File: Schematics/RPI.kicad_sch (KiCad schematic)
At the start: 7 parts, among them J1 RPi GPIO, U2 24LC256

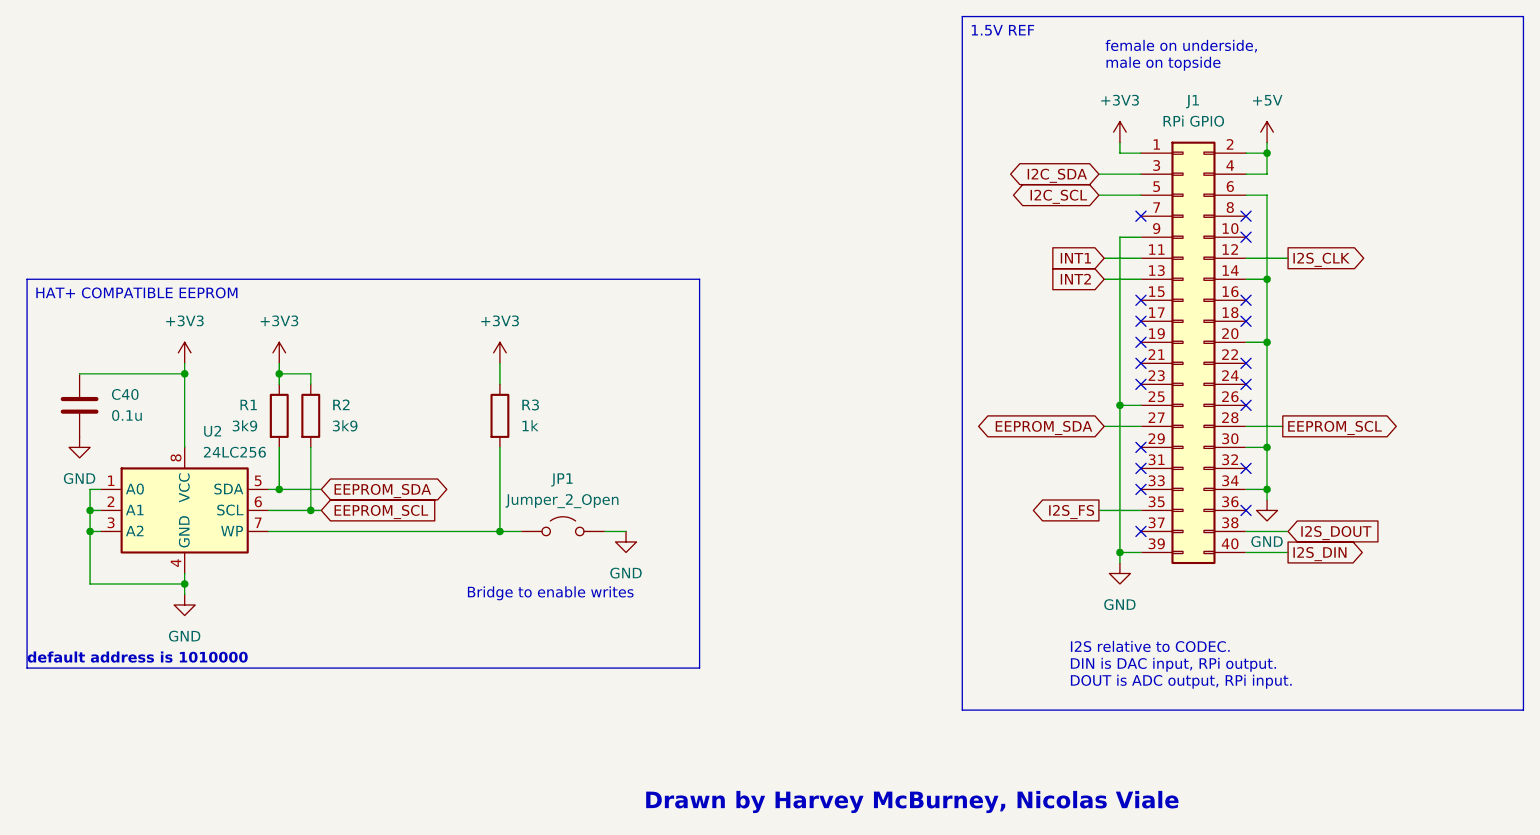
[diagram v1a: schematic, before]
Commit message: Tidied up Schematic
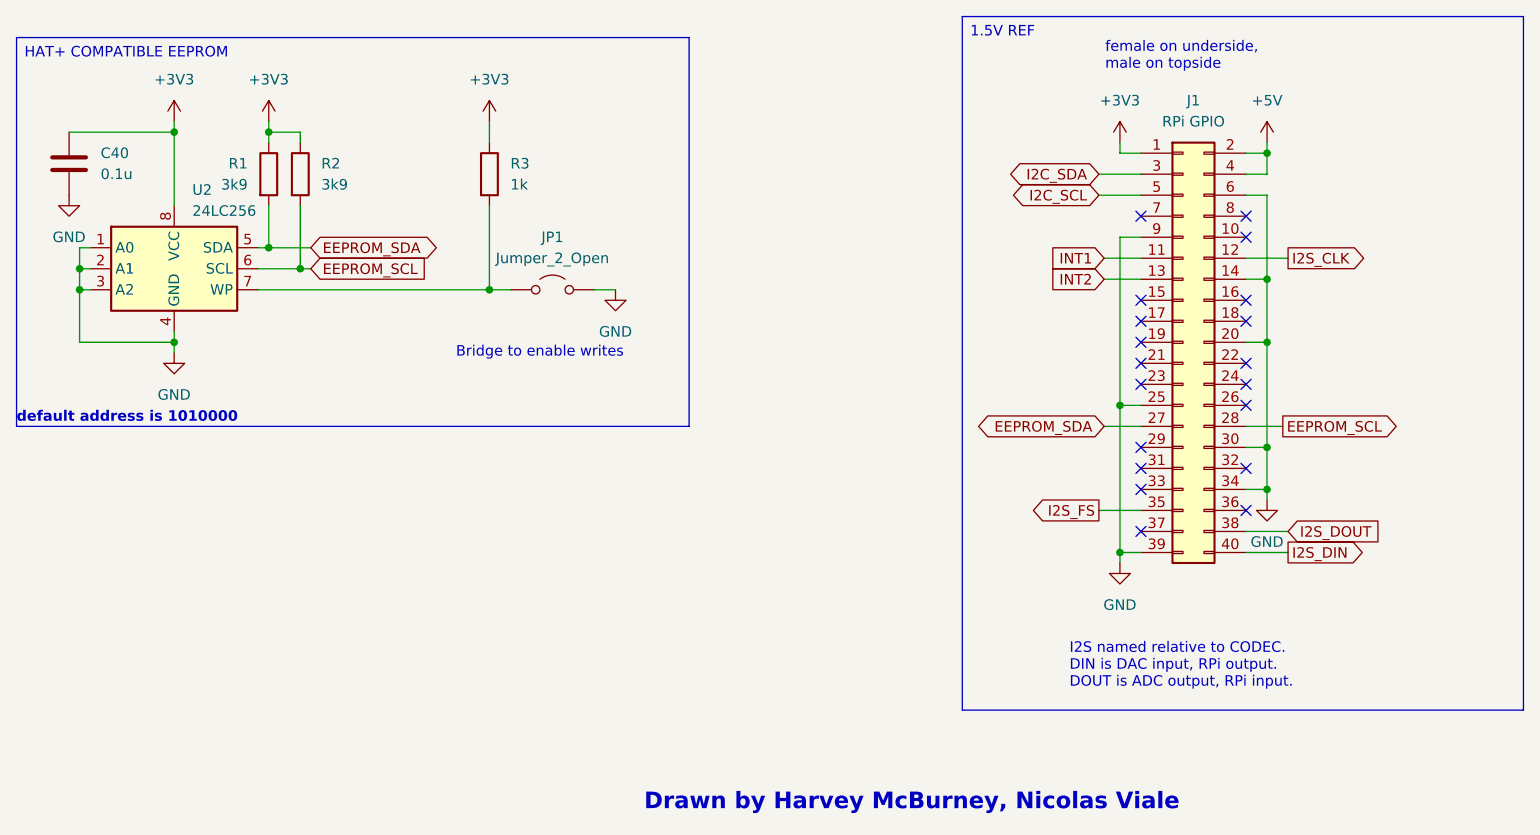
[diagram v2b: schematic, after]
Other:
- note added: "I2S named relative to CODEC. DIN is DAC input, RPi output. DOUT is ADC output, RPi input."
- note removed: "I2S relative to CODEC. DIN is DAC input, RPi output. DOUT is ADC output, RPi input."
- moved on the sheet: C40, JP1, R1, R2, R3, U2
